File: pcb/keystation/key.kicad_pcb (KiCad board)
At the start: 2 copper layers, 66 x 55.9 mm, 25 parts, among them J1 Button, J2 speaker, J3 Vin, J4 AVR-ISP-6, Q1 IRF540N, U2 LM741, U3 LM1117MP-3.3, U4 ATtiny84A-SS

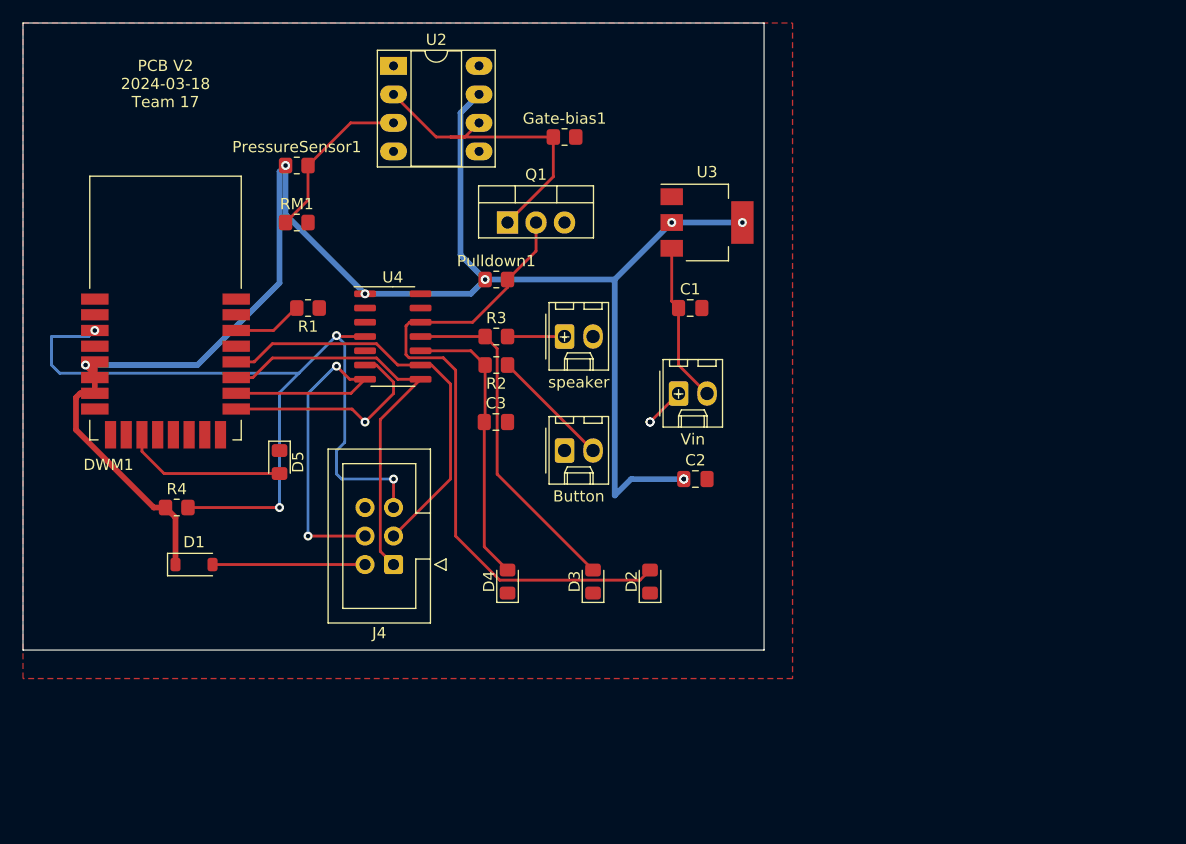
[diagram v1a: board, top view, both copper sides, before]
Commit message: dish pcb updated
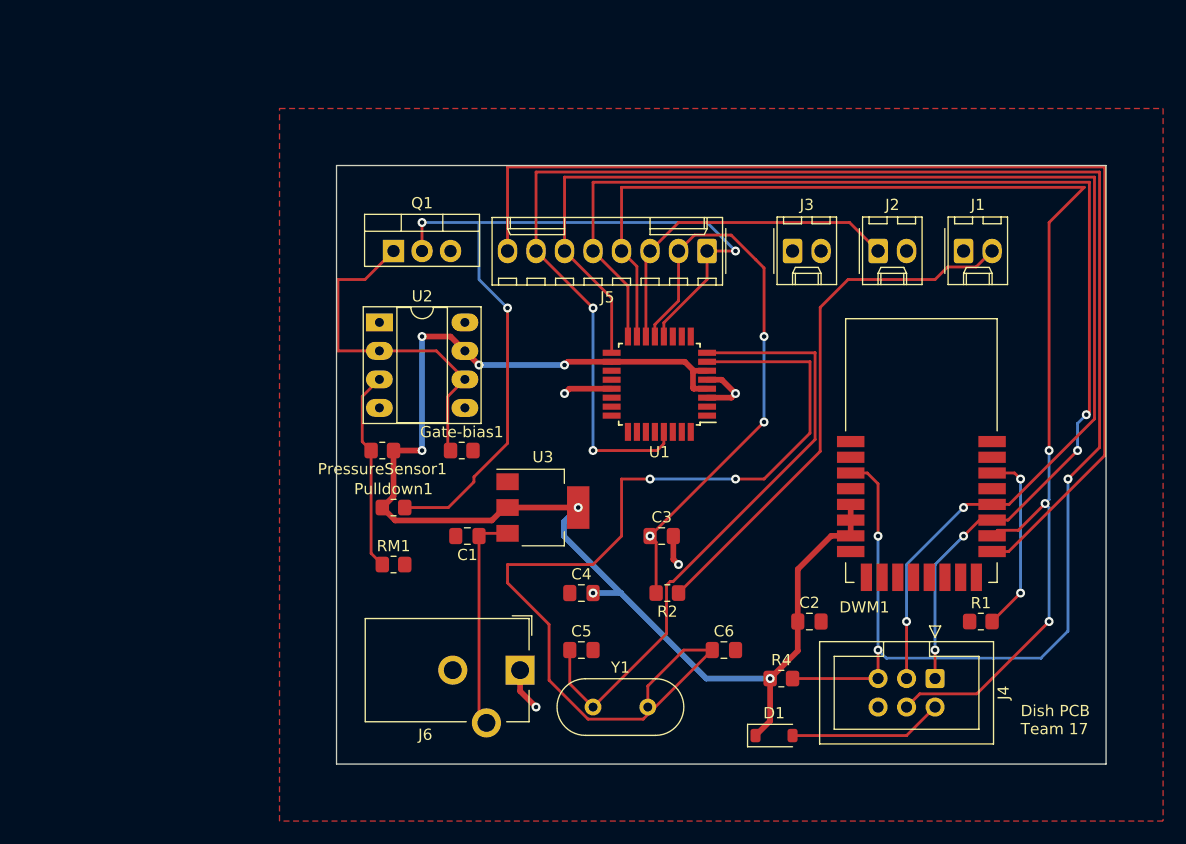
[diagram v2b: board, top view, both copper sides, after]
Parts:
- removed D2, D3, D4, D5: LED, LED_SMD:LED_0805_2012Metric_Pad1.15x1.40mm_HandSolder
- removed R3: 1k, Resistor_SMD:R_0805_2012Metric_Pad1.20x1.40mm_HandSolder
- removed U4: ATtiny84A-SS, Package_SO:SOIC-14_3.9x8.7mm_P1.27mm
- added C4: 1uF, Capacitor_SMD:C_0805_2012Metric_Pad1.18x1.45mm_HandSolder, F.Cu at (146.3, 91.4)
- added C5: 22p, Capacitor_SMD:C_0805_2012Metric_Pad1.18x1.45mm_HandSolder, F.Cu at (146.3, 96.5)
- added C6: 22p, Capacitor_SMD:C_0805_2012Metric_Pad1.18x1.45mm_HandSolder, F.Cu at (159.0, 96.5)
- added J5: Conn_01x08, Connector_Molex:Molex_KK-254_AE-6410-08A_1x08_P2.54mm_Vertical, F.Cu at (157.5, 61.0)
- added J6: Barrel_Jack_Switch, Connector_BarrelJack:BarrelJack_CUI_PJ-102AH_Horizontal, F.Cu at (140.8, 98.3)
- added U1: ATmega328-A, Package_QFP:TQFP-32_7x7mm_P0.8mm, F.Cu at (153.2, 72.8)
- added Y1: 16MHz, Crystal:Crystal_HC49-U_Vertical, F.Cu at (147.3, 101.6)
- moved DWM1 68.5 mm to (176.6, 78.7)
- moved R1 66.2 mm to (181.9, 94.0), turned to 0 degrees
- moved R4 56.0 mm to (164.1, 99.1)
- moved D1 53.9 mm to (163.4, 104.1)
- moved J4 49.3 mm to (177.8, 99.1), turned to -90 degrees
- moved J1 39.8 mm to (180.3, 61.0)
- moved RM1 31.7 mm to (129.5, 88.9)
- moved Gate-bias1 29.4 mm to (135.6, 78.7)
- moved U3 29.3 mm to (142.8, 83.8)
- moved J2 29.0 mm to (172.7, 61.0)
- moved C1 28.4 mm to (136.1, 86.4), turned to 180 degrees
- moved PressureSensor1 26.5 mm to (128.5, 78.7), turned to 180 degrees
- moved R2 25.4 mm to (153.9, 91.4)
- moved U2 22.9 mm to (128.3, 67.3)
- moved Pulldown1 22.3 mm to (129.5, 83.8)
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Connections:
- net /RST renamed /RESET
- C1 pad 1: Net-(J3-Pin_2) -> Net-(U3-VI)
- DWM1 pad 11: Net-(D5-A) -> unconnected-(DWM1-GPIO4/EXTPA-Pad11)
- DWM1 pad 22: /interrupt -> unconnected-(DWM1-IRQ/GPIO8-Pad22)
- J2 pad 1: Net-(J2-Pin_1) -> /alarm
- R1 pad 2: /interrupt -> unconnected-(DWM1-IRQ/GPIO8-Pad22)
- U3 pad 3: Net-(J3-Pin_2) -> Net-(U3-VI)
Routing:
- net /RESET: track 79.5 -> 173.2 mm, vias 4 -> 5
- net Net-(U1-XTAL1/PB6): track 0.00 -> 89.6 mm, vias 0 -> 2
- net /SCK: track 36.9 -> 118.5 mm, vias 0 -> 2
- net /MOSI: track 36.4 -> 117.2 mm, vias 2 -> 3
- net /Csn: track 20.8 -> 101.0 mm, vias 1 -> 0
- net /MISO: track 37.1 -> 110.7 mm, vias 0 -> 4
- net Net-(U1-XTAL2/PB7): track 0.00 -> 55.5 mm
- net Net-(J1-Pin_2): track 10.8 -> 48.1 mm
- net +3.3V: track 153.3 -> 120.7 mm, vias 8 -> 7
- net /button: track 25.4 -> 51.9 mm, vias 0 -> 3
- net Net-(U3-VI): track 0.00 -> 19.6 mm
- net unconnected-(DWM1-IRQ/GPIO8-Pad22): track 0.00 -> 16.5 mm, vias 0 -> 2
- net /confirmation: track 59.8 -> 75.8 mm, vias 0 -> 3
- net Net-(D5-A): track 14.6 -> 0.00 mm
- net Net-(J3-Pin_2): track 14.2 -> 0.00 mm
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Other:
- board size 66 x 55.9 mm -> 68.6 x 53.3 mm
- board text added: "Dish PCB Team 17"
- board text removed: "PCB V2 2024-03-18 Team 17"
